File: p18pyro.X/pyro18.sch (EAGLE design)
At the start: 12 parts, among them U1 TPIC6B595PTH, U2 TPIC6B595PTH, X1 332-10, X2 332-10, X3 332-10, X4 332-10, X5 22-23-2041, X7 22-23-2021

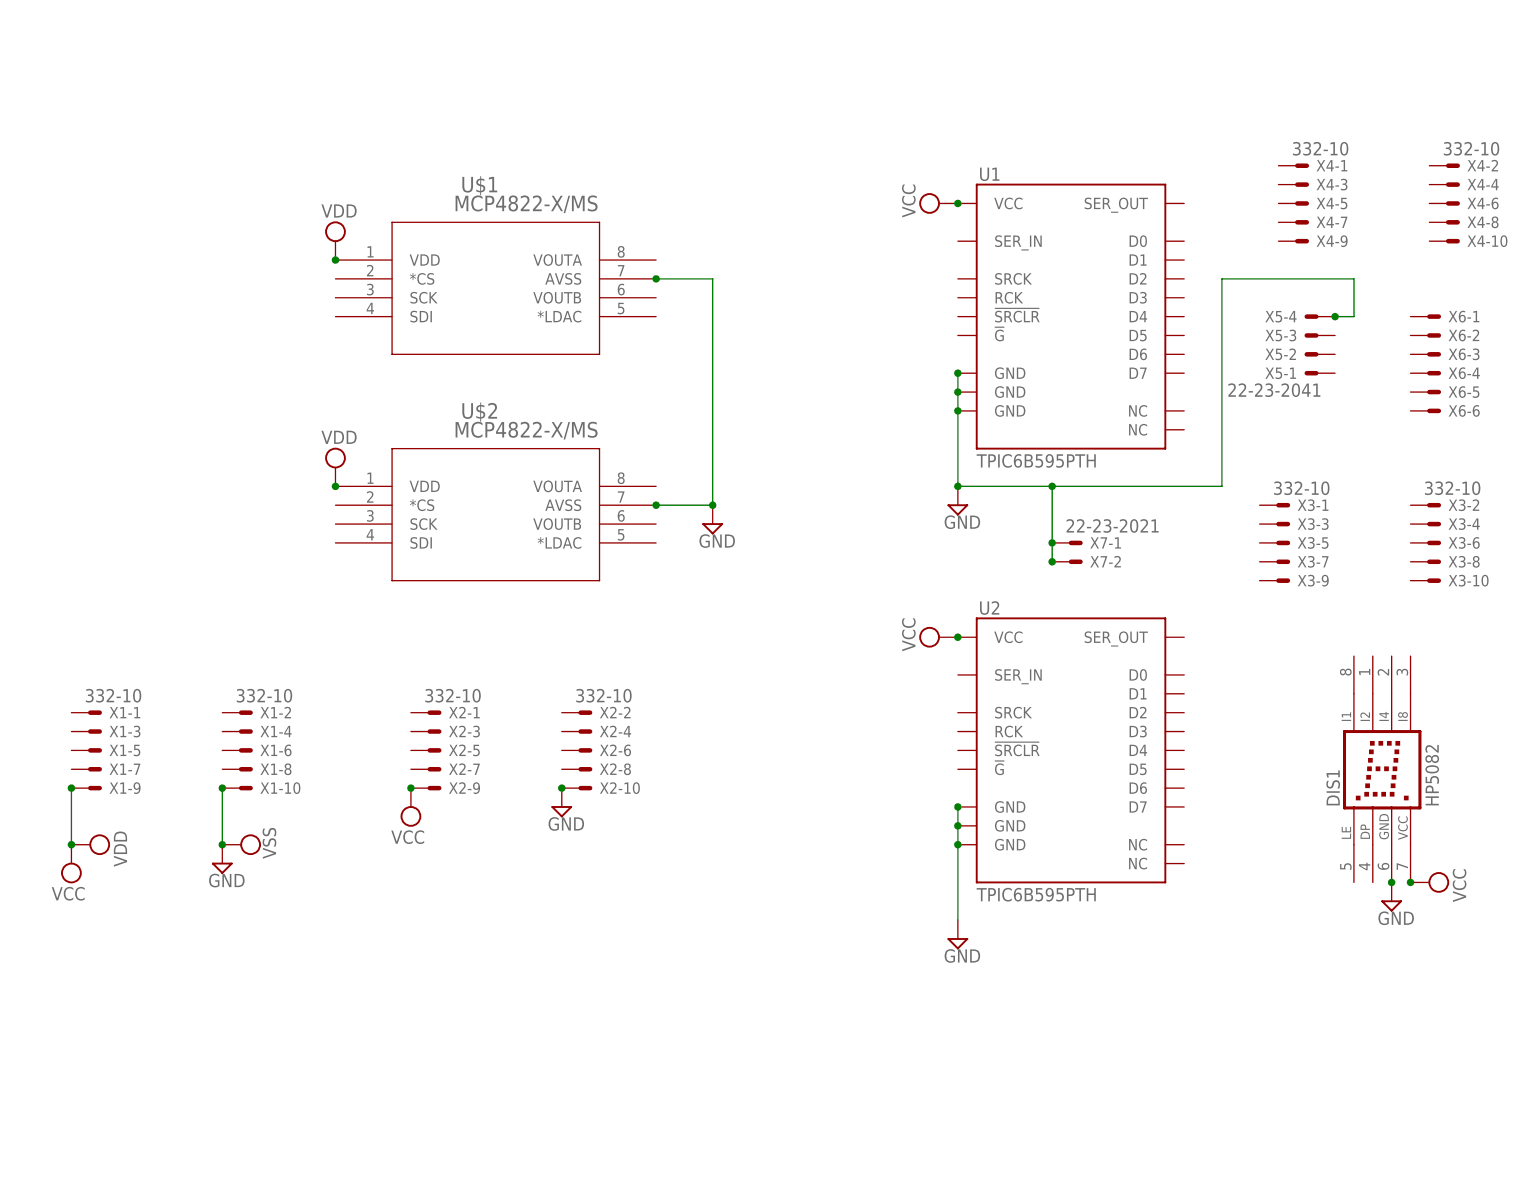
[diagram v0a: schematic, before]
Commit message: update
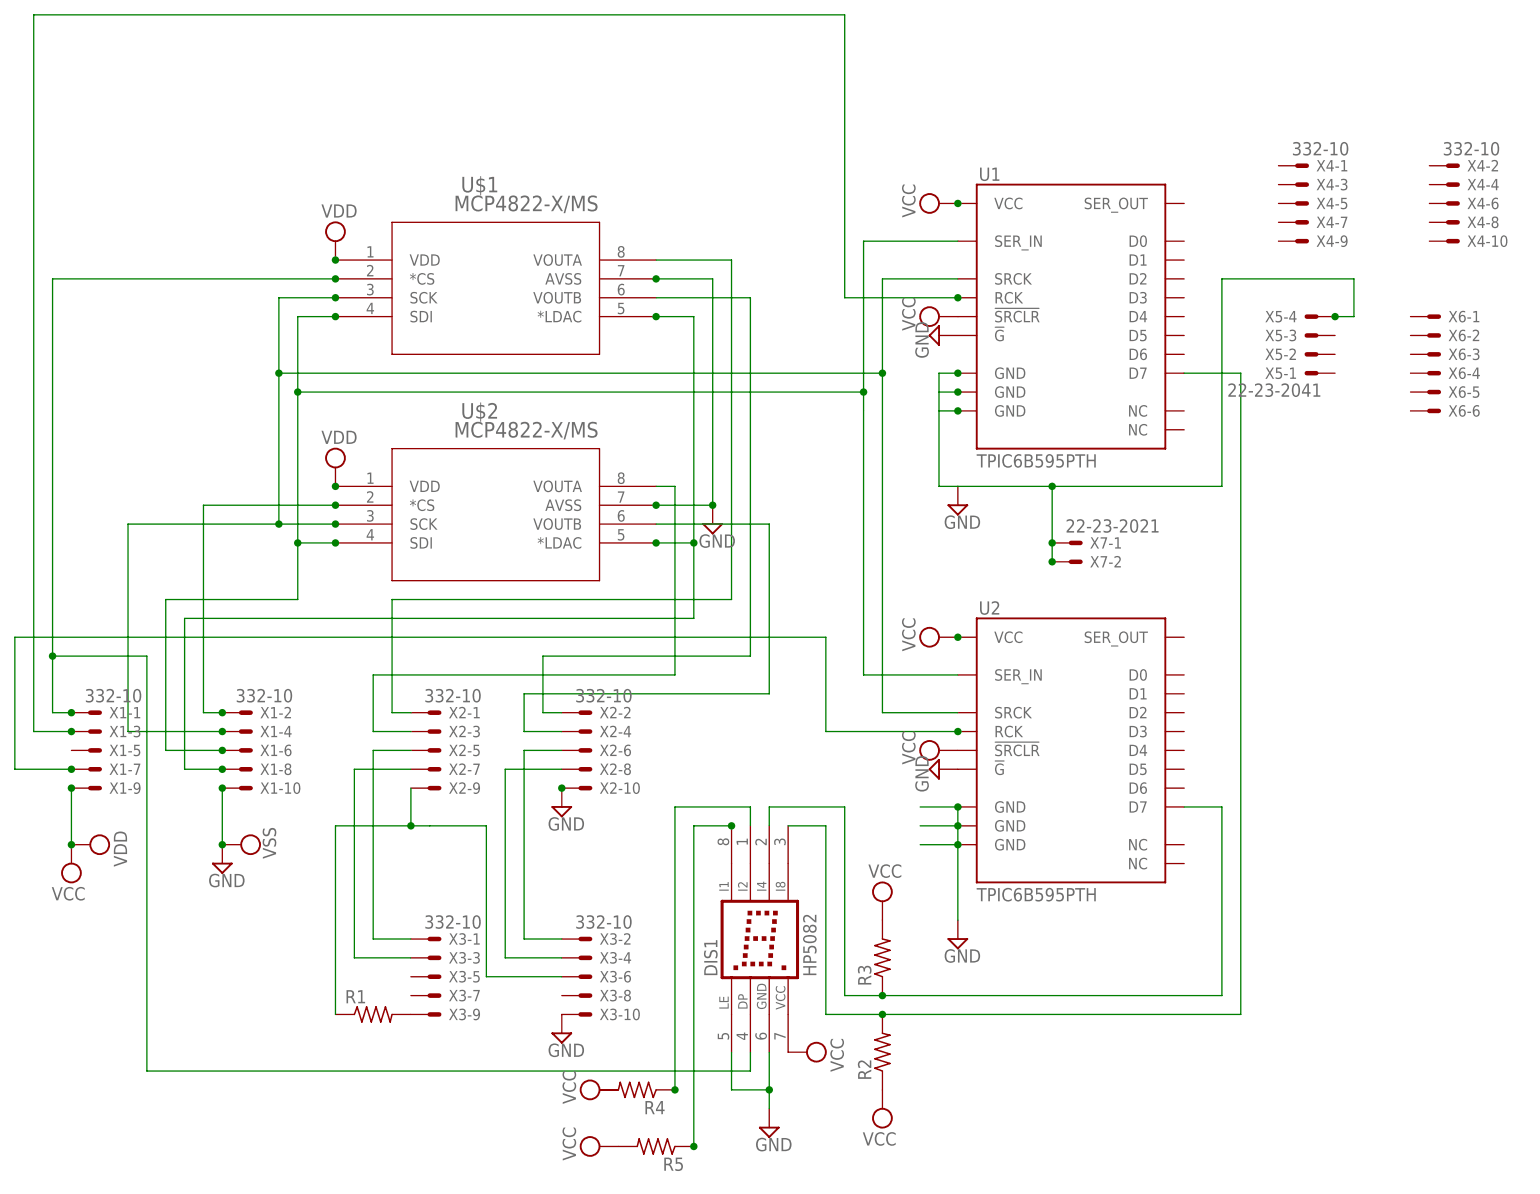
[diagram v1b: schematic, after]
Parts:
- added R1, R2, R3, R4, R5: (no value), resistor:R-US_0207/2V
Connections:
- removed net N$8: U2.GND@11
- removed net N$9: U2.GND@19
- new net N$1: DIS1.DP, U$1.*CS, X1-1.S
- new net N$10: U$1.VOUTB, X2-2.S
- new net N$12: U$1.SDI, U$2.SDI, U1.SER_IN, U2.SER_IN, X1-6.S
- new net N$13: U$2.VOUTA, X2-3.S
- new net N$14: U1.RCK, X1-3.S
- new net N$15: U2.RCK, X1-7.S
- new net N$16: U$2.VOUTB, X2-4.S
- new net N$17: X2-5.S, X3-1.S
- new net N$18: X2-6.S, X3-2.S
- new net N$19: X2-7.S, X3-3.S
- new net N$2: U$2.*CS, X1-2.S
- new net N$20: X2-8.S, X3-4.S
- new net N$21: R1.1, X2-9.S, X3-6.S
- new net N$22: R1.2, X3-9.S
- new net N$23: DIS1.I4, R3.1, U2.D7
- new net N$24: DIS1.I8, R2.2, U1.D7
- new net N$26: DIS1.I1, R5.1
- new net N$27: DIS1.I2, R4.1
- new net N$3: U$1.*LDAC, U$2.*LDAC, X1-8.S
- new net N$4: U$1.VOUTA, X2-1.S
- new net N$7: U$1.SCK, U$2.SCK, U1.SRCK, U2.SRCK, X1-4.S
- net GND: now also DIS1.LE, U1.!G, U2.!G, U2.GND@11, U2.GND@19, X3-10.S
- net VCC: now also R2.1, R3.2, R5.2, U1.!SRCLR, U2.!SRCLR; no longer X2-9.S
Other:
- moved on the sheet: DIS1, X3-1, X3-10, X3-2, X3-3, X3-4, X3-5, X3-6, X3-7, X3-8, X3-9
